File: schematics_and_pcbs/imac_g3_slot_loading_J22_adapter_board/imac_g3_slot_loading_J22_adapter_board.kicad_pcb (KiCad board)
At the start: 2 copper layers, 65 x 30 mm, 12 parts, among them J1 Conn_02x13_Odd_Even, J2 Screw_Terminal_01x10, J3 AudioJack3, J4 Conn_02x03_Odd_Even

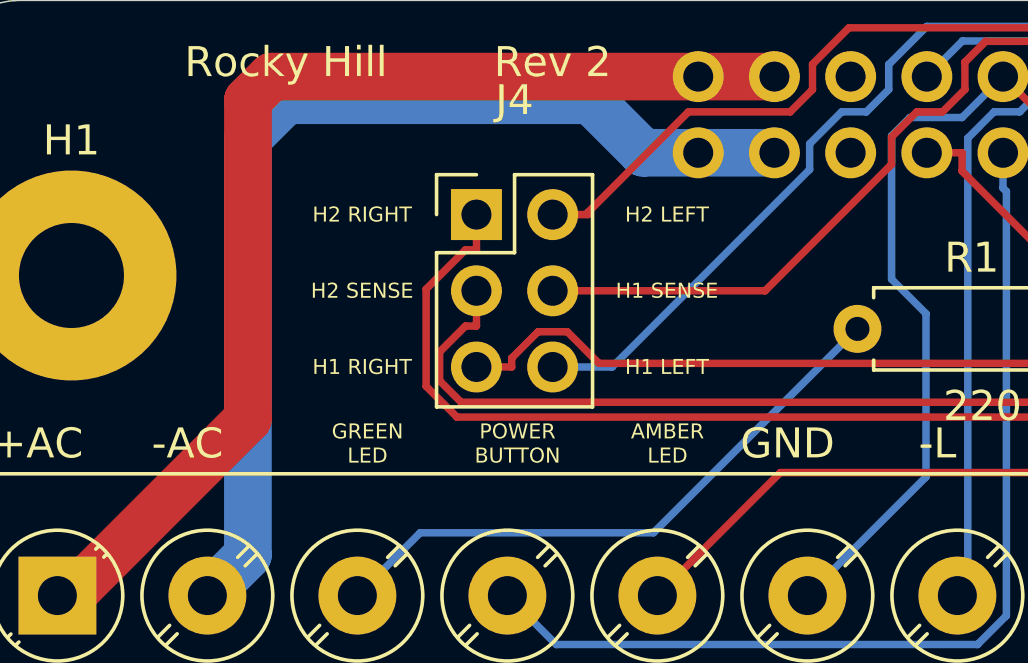
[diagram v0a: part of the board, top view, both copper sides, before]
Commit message: updated silkscreen to make it more readable
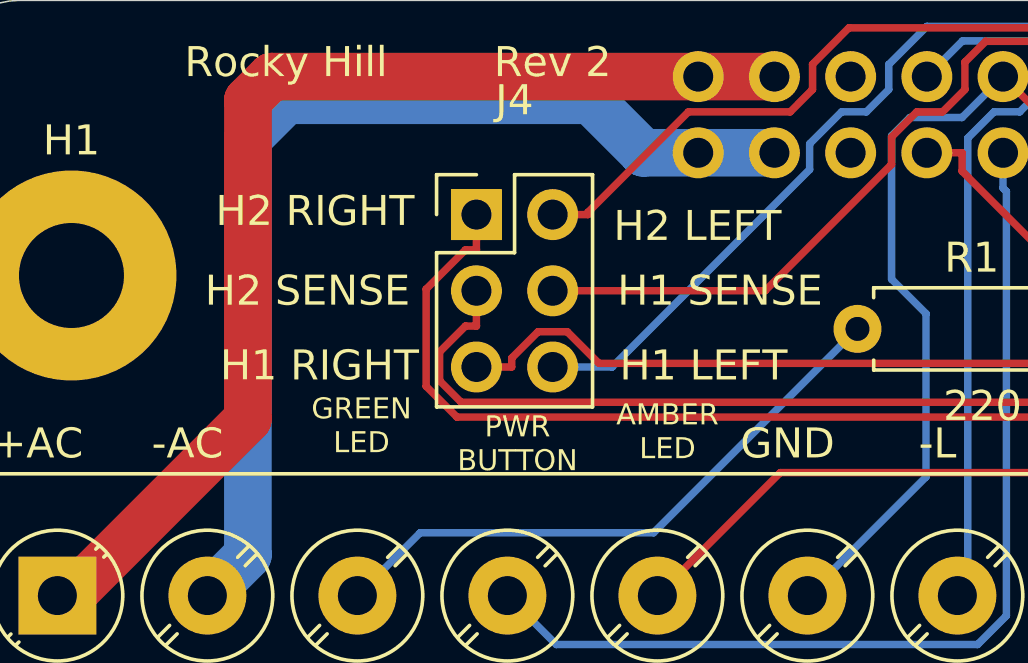
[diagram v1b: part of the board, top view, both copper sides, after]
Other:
- board text added: "PWR BUTTON"
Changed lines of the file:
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@@
   )
   (layers
-    (0 F.Cu signal hide)
+    (0 F.Cu signal)
     (31 B.Cu signal)
     (32 B.Adhes user)
@@
     (effects (font (size 1 1) (thickness 0.15)))
   )
-  (gr_text "GREEN\nLED" (at 120.04 101.64) (layer F.SilkS)
-    (effects (font (size 0.5 0.5) (thickness 0.1)))
-  )
-  (gr_text "POWER\nBUTTON" (at 125.04 101.64) (layer F.SilkS)
-    (effects (font (size 0.5 0.5) (thickness 0.1)))
-  )
-  (gr_text "AMBER\nLED" (at 130.04 101.64) (layer F.SilkS)
-    (effects (font (size 0.5 0.5) (thickness 0.1)))
+  (gr_text "GREEN\nLED" (at 119.84 101.04) (layer F.SilkS)
+    (effects (font (size 0.7 0.7) (thickness 0.15)))
+  )
+  (gr_text "PWR\nBUTTON" (at 125.04 101.64) (layer F.SilkS)
+    (effects (font (size 0.7 0.7) (thickness 0.15)))
+  )
+  (gr_text "AMBER\nLED" (at 130.04 101.24) (layer F.SilkS)
+    (effects (font (size 0.7 0.7) (thickness 0.15)))
   )
   (gr_text GND (at 134.04 101.64) (layer F.SilkS)
@@
     (effects (font (size 1 1) (thickness 0.15)))
   )
-  (gr_text "H2 LEFT" (at 130.022 94.008) (layer F.SilkS)
-    (effects (font (size 0.5 0.5) (thickness 0.1)))
-  )
-  (gr_text "H1 SENSE" (at 130.022 96.548) (layer F.SilkS)
-    (effects (font (size 0.5 0.5) (thickness 0.1)))
-  )
-  (gr_text "H2 RIGHT" (at 119.862 94.008) (layer F.SilkS)
-    (effects (font (size 0.5 0.5) (thickness 0.1)))
-  )
-  (gr_text "H2 SENSE" (at 119.862 96.548) (layer F.SilkS)
-    (effects (font (size 0.5 0.5) (thickness 0.1)))
-  )
-  (gr_text "H1 RIGHT" (at 119.862 99.088) (layer F.SilkS)
-    (effects (font (size 0.5 0.5) (thickness 0.1)))
-  )
-  (gr_text "H1 LEFT" (at 130.022 99.088) (layer F.SilkS)
-    (effects (font (size 0.5 0.5) (thickness 0.1)))
+  (gr_text "H2 LEFT" (at 131.04 94.39) (layer F.SilkS)
+    (effects (font (size 1 1) (thickness 0.15)))
+  )
+  (gr_text "H1 SENSE" (at 131.79 96.548) (layer F.SilkS)
+    (effects (font (size 1 1) (thickness 0.15)))
+  )
+  (gr_text "H2 RIGHT" (at 118.29 93.89) (layer F.SilkS)
+    (effects (font (size 1 1) (thickness 0.15)))
+  )
+  (gr_text "H2 SENSE" (at 118.04 96.548) (layer F.SilkS)
+    (effects (font (size 1 1) (thickness 0.15)))
+  )
+  (gr_text "H1 RIGHT" (at 118.44 99.04) (layer F.SilkS)
+    (effects (font (size 1 1) (thickness 0.15)))
+  )
+  (gr_text "H1 LEFT" (at 131.24 99.04) (layer F.SilkS)
+    (effects (font (size 1 1) (thickness 0.15)))
   )
   (gr_line (start 112.242 114.328) (end 105.892 114.328) (layer F.SilkS) (width 0.12))
